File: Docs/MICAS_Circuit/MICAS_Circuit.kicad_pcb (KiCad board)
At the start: 2 copper layers, 76.8 x 84.5 mm, 34 parts, among them Q1 BD140, Q2 BD140, U1 ESP32_DevKit_V1_DOIT

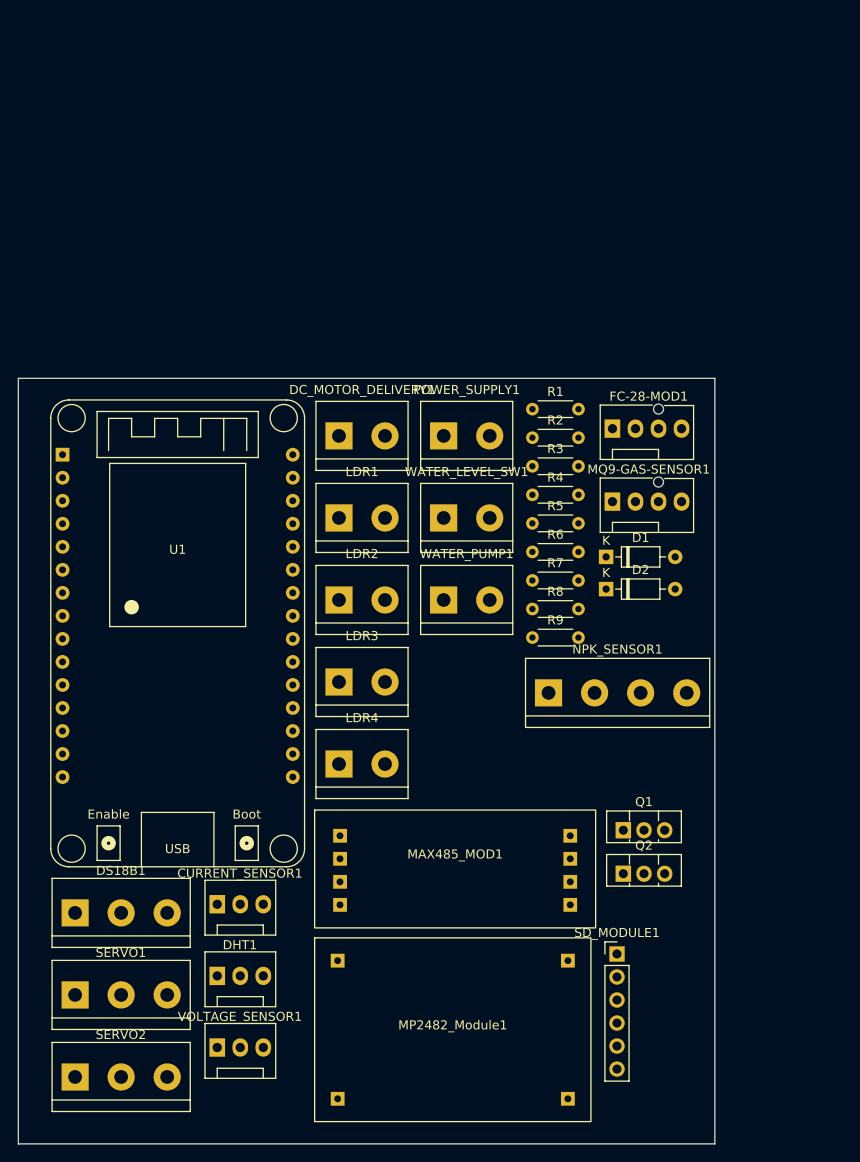
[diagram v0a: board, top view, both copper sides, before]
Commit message: update repository with circuit data
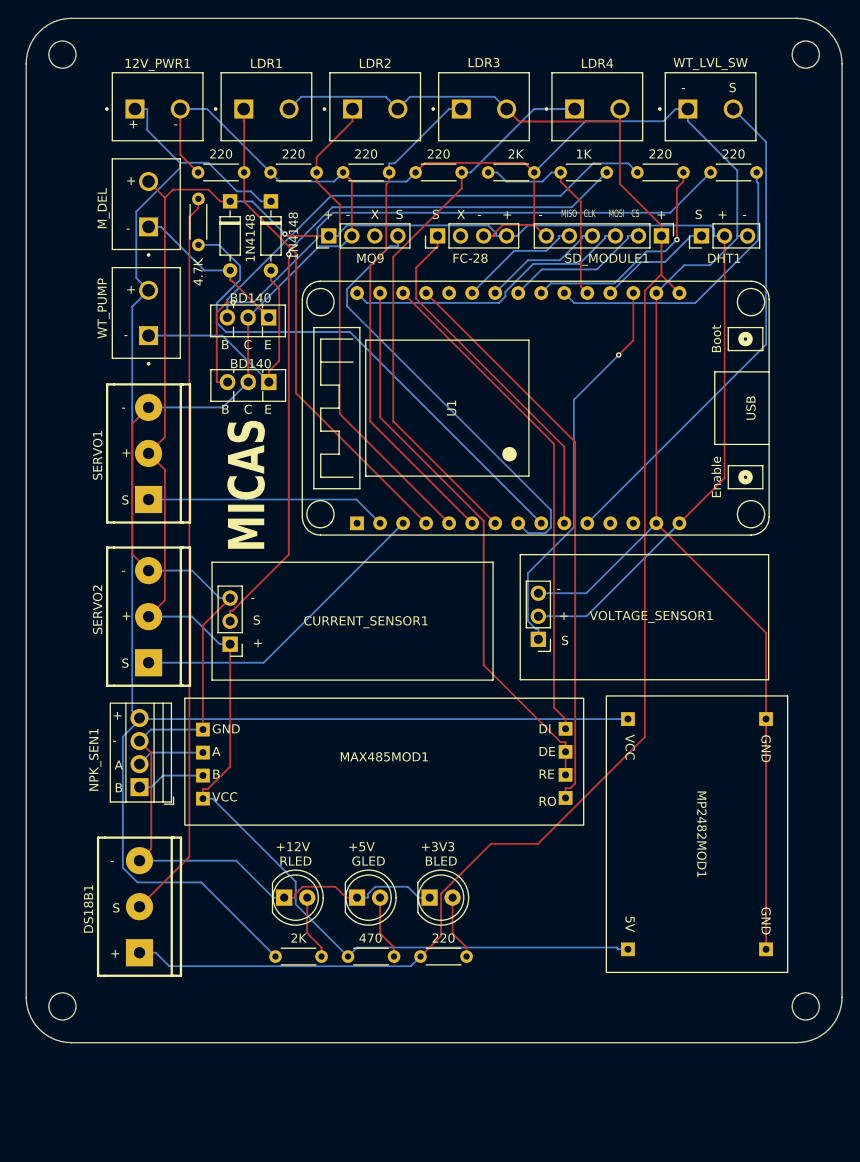
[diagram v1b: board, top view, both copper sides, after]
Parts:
- removed DC_MOTOR_DELIVERY1, POWER_SUPPLY1, WATER_LEVEL_SW1, WATER_PUMP1: Screw_Terminal_01x02, TerminalBlock:TerminalBlock_bornier-2_P5.08mm
- removed FC-28-MOD1, MQ9-GAS-SENSOR1: FC-28-MOD, Connector:FanPinHeader_1x04_P2.54mm_Vertical
- removed MAX485_MOD1: ~, MAX485_Module:MAX485_MODULE
- removed MP2482_Module1: ~, MP2482_Module:MP2482_Module
- removed NPK_SENSOR1: Screw_Terminal_01x04, TerminalBlock:TerminalBlock_bornier-4_P5.08mm
- added 12V_PWR1: Screw_Terminal_01x02, KF301-2P:KF301-2P, F.Cu at (48.4, 39.5)
- added D3: RLED, LED_THT:LED_D5.0mm_FlatTop, F.Cu at (62.3, 126.5)
- added D4: GLED, LED_THT:LED_D5.0mm_FlatTop, F.Cu at (70.4, 126.5)
- added D5: BLED, LED_THT:LED_D5.0mm_FlatTop, F.Cu at (78.4, 126.5)
- added FC-28: FC-28-MOD, Connector_PinHeader_2.54mm:PinHeader_1x04_P2.54mm_Vertical, F.Cu at (79.3, 53.5)
- added MAX485MOD1: ~, MAX485_Module:MAX485_MOD, F.Cu at (73.4, 111.5)
- added MP2482MOD1: ~, MP2482_Module:MP2482_MOD, F.Cu at (107.9, 119.5)
- added MQ9: FC-28-MOD, Connector_PinHeader_2.54mm:PinHeader_1x04_P2.54mm_Vertical, F.Cu at (67.3, 53.5)
- added M_DEL: Screw_Terminal_01x02, KF301-2P:KF301-2P, F.Cu at (47.4, 50.0)
- added NPK_SEN1: Screw_Terminal_01x04, TerminalBlock:TerminalBlock_Xinya_XY308-2.54-4P_1x04_P2.54mm_Horizontal, F.Cu at (46.4, 114.3)
- added R10: 2K, Resistor_THT:R_Axial_DIN0204_L3.6mm_D1.6mm_P5.08mm_Horizontal, F.Cu at (61.4, 133.0)
- added R11: 470, Resistor_THT:R_Axial_DIN0204_L3.6mm_D1.6mm_P5.08mm_Horizontal, F.Cu at (69.4, 133.0)
- added R12: 220, Resistor_THT:R_Axial_DIN0204_L3.6mm_D1.6mm_P5.08mm_Horizontal, F.Cu at (77.4, 133.0)
- added WT_LVL_SW: Screw_Terminal_01x02, KF301-2P:KF301-2P, F.Cu at (109.4, 39.5)
- added WT_PUMP: Screw_Terminal_01x02, KF301-2P:KF301-2P, F.Cu at (47.4, 62.0)
- CURRENT_SENSOR1, DHT1, VOLTAGE_SENSOR1: footprint Connector:FanPinHeader_1x03_P2.54mm_Vertical -> Connector_PinHeader_2.54mm:PinHeader_1x03_P2.54mm_Vertical
- DS18B1, SERVO1, SERVO2: footprint TerminalBlock:TerminalBlock_bornier-3_P5.08mm -> KF301-3P:KF301-3P
- LDR1, LDR2, LDR3, LDR4: footprint TerminalBlock:TerminalBlock_bornier-2_P5.08mm -> KF301-2P:KF301-2P
- U1: footprint esp32_devkit_v1_doit:esp32_devkit_v1_doit -> ESP3_DEVKIT_30PIN:esp32_devkit_v1_doit
- moved DHT1 97.6 mm to (108.4, 53.5), turned to 90 degrees
- moved SD_MODULE1 79.4 mm to (104.0, 53.5), turned to -90 degrees
- moved LDR4 77.7 mm to (96.9, 39.5)
- moved Q1 68.8 mm to (60.6, 62.5), turned to 180 degrees
- moved Q2 66.9 mm to (60.7, 69.6), turned to 180 degrees
- moved LDR3 65.2 mm to (84.4, 39.5)
- moved SERVO1 60.3 mm to (47.4, 77.5), turned to 90 degrees
- moved VOLTAGE_SENSOR1 57.3 mm to (90.4, 98.0), turned to 180 degrees
- moved D1 57.1 mm to (56.4, 49.7), turned to -90 degrees
- moved D2 56.5 mm to (60.9, 49.7), turned to -90 degrees
- moved R9 54.9 mm to (109.4, 46.5)
- moved LDR2 54.3 mm to (72.4, 39.5)
- moved SERVO2 51.4 mm to (47.4, 95.5), turned to 90 degrees
- moved R8 49.5 mm to (101.3, 46.5)
- moved R5 48.0 mm to (52.9, 54.5), turned to 90 degrees
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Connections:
- net 3.3 VDC renamed +3V3
- net 5 VDC renamed +5V
- D2 pad 1: 12 VDC -> +12V
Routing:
- net GND: track 0.00 -> 354.2 mm
- net +5V: track 0.00 -> 256.4 mm, vias 0 -> 1
- net +3V3: track 0.00 -> 183.7 mm
- net +12V: track 0.00 -> 177.5 mm
- net Net-(CURRENT_SENSOR1-Pin_2): track 0.00 -> 82.3 mm, vias 0 -> 1
- net Net-(DS18B1-Pin_2): track 0.00 -> 80.8 mm
- net Net-(Q2-B): track 0.00 -> 70.4 mm, vias 0 -> 1
- net RO_SIGNAL: track 0.00 -> 63.3 mm
- net RE_SIGNAL: track 0.00 -> 61.9 mm
- net LDR4_SIGNAL: track 0.00 -> 61.8 mm
- net DS18B20_SIGNAL: track 0.00 -> 57.9 mm
- net LDR3_SIGNAL: track 0.00 -> 55.7 mm
- net DI_SIGNAL: track 0.00 -> 55.5 mm
- net WATER_LEVEL_SIGNAL: track 0.00 -> 55.4 mm
- net LDR1_SIGNAL: track 0.00 -> 54.0 mm
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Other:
- board size 76.8 x 84.5 mm -> 90 x 113 mm
- board text added: "+"
- board text added: "+12V"
- board text added: "+3V3"
- board text added: "+5V"
- board text added: "-"
- board text added: "A"
- board text added: "B"
- board text added: "C"
- board text added: "CLK"
- board text added: "CS"
- board text added: "DS18B1"
- board text added: "E"
- board text added: "MICAS"
- board text added: "MISO"
- board text added: "MOSI"
- board text added: "S"
- board text added: "SERVO1"
- board text added: "SERVO2"
- board text added: "X"
